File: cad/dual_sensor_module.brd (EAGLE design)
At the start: 28.2 x 40 mm, 14 parts, among them IC1 MCP602SN, IC2 TC7660DIL8

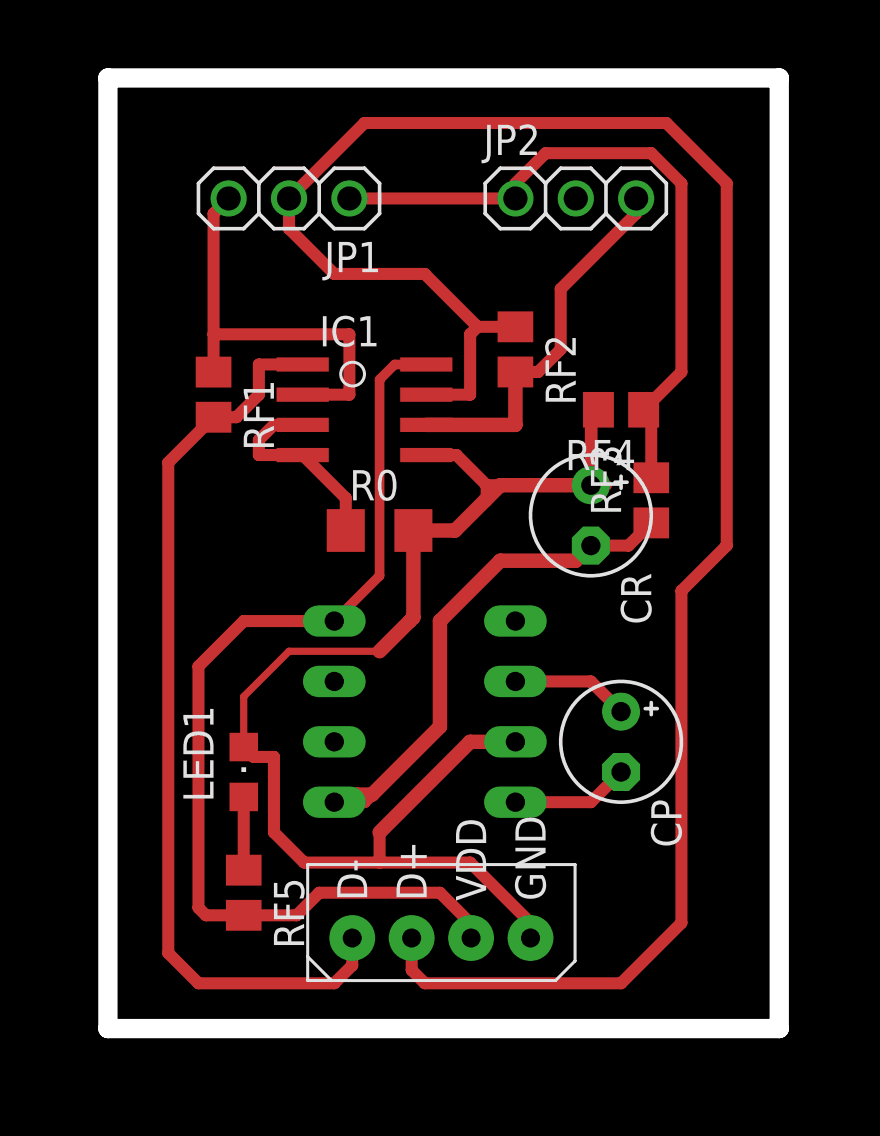
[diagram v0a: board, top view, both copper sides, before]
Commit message: update pcb files
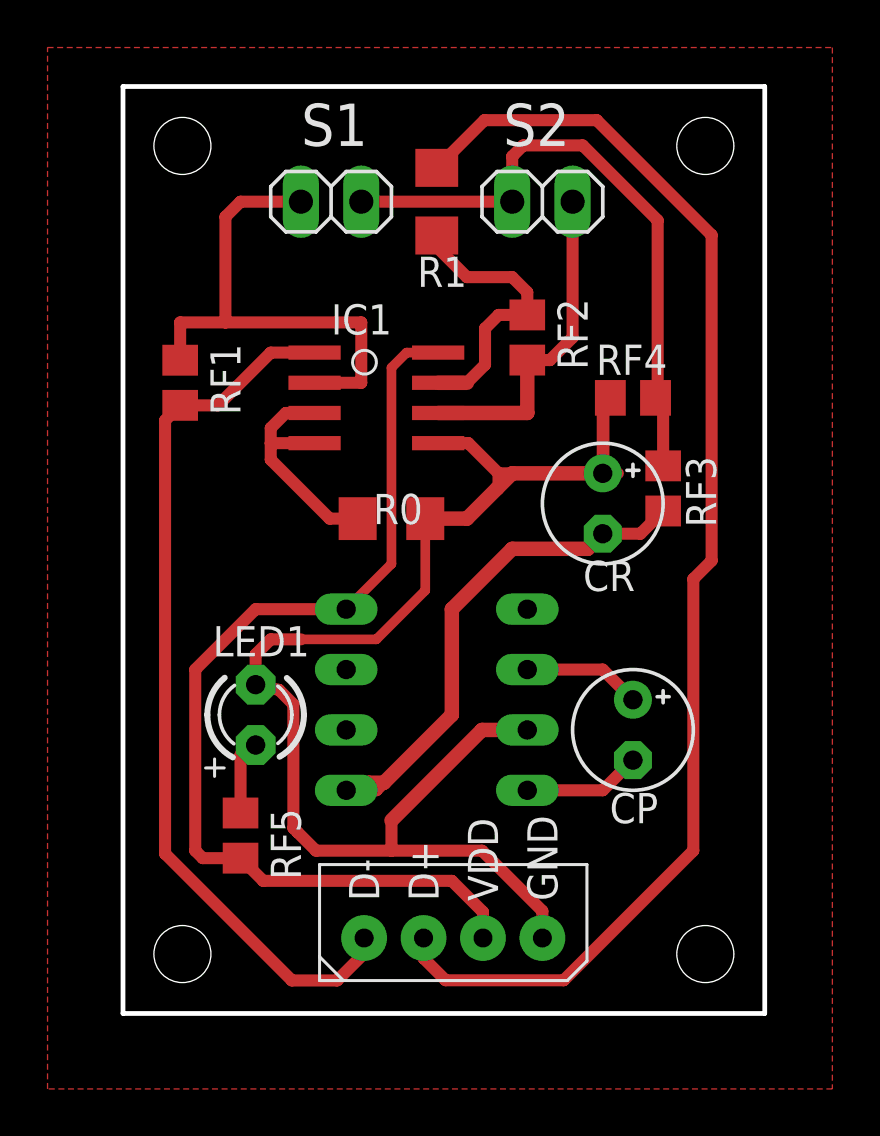
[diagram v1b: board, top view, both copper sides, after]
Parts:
- removed JP1, JP2: (no value), adafruit:1X03
- added JP3, JP4: (no value), pinhead:1X02
- added R1: (no value), rcl:R1206
- LED1: device adafruit:CHIPLED_0805 -> adafruit:LED3MM
- moved LED1 2.46 mm to (5.58, 12.6), turned to 90 degrees
- moved RF5 2.41 mm to (4.95, 7.49)
- moved RF1 1.49 mm to (2.40, 26.5)
- moved CP 0.71 mm to (21.5, 11.9)
- moved CR 0.71 mm to (20.2, 21.5)
- moved IC1 0.71 mm to (10.7, 25.9)
- moved IC2 0.71 mm to (13.2, 13.2)
- moved R0 0.71 mm to (11.3, 20.8)
- moved RF2 0.71 mm to (17.0, 28.4)
- moved RF3 0.71 mm to (22.7, 22.1)
- moved RF4 0.71 mm to (21.5, 25.9)
- moved U$1 0.50 mm to (17.6, 3.17)
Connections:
- new net VOUT22: IC1.7, R1.1, RF2.1
- net GND: now also LED1.K; no longer LED1.C
- net N$52: now also JP4.2; no longer JP1.3
- net N$82: now also JP3.2; no longer JP2.3
- net VOUT2: now also R1.2; no longer IC1.7, RF2.1
- net VT: now also JP3.1, JP4.1; no longer JP1.1, JP2.1
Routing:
- net VOUT2: track 84.0 -> 55.5 mm
- net VOUT22: track 0.00 -> 11.9 mm
- net N$52: track 17.8 -> 21.6 mm
- net VT: track 29.1 -> 26.6 mm
- net GND: track 73.5 -> 75.7 mm
- net N$82: track 15.9 -> 14.0 mm
- net VOUT1: track 38.5 -> 37.4 mm
- net +5V: track 43.0 -> 42.5 mm
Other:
- board size 28.2 x 40 mm -> 27 x 39 mm
- board text added: "S1"
- board text added: "S2"
